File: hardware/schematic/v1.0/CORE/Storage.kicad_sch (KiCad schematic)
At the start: 43 parts, among them J12 USB_C_Receptacle_USB2.0_16P, U1 TXS02612RTWR, U12 FT2232HL, U3 SD_Card, U6 93LC56BT-I_OT, X1 X322512MSB4SI

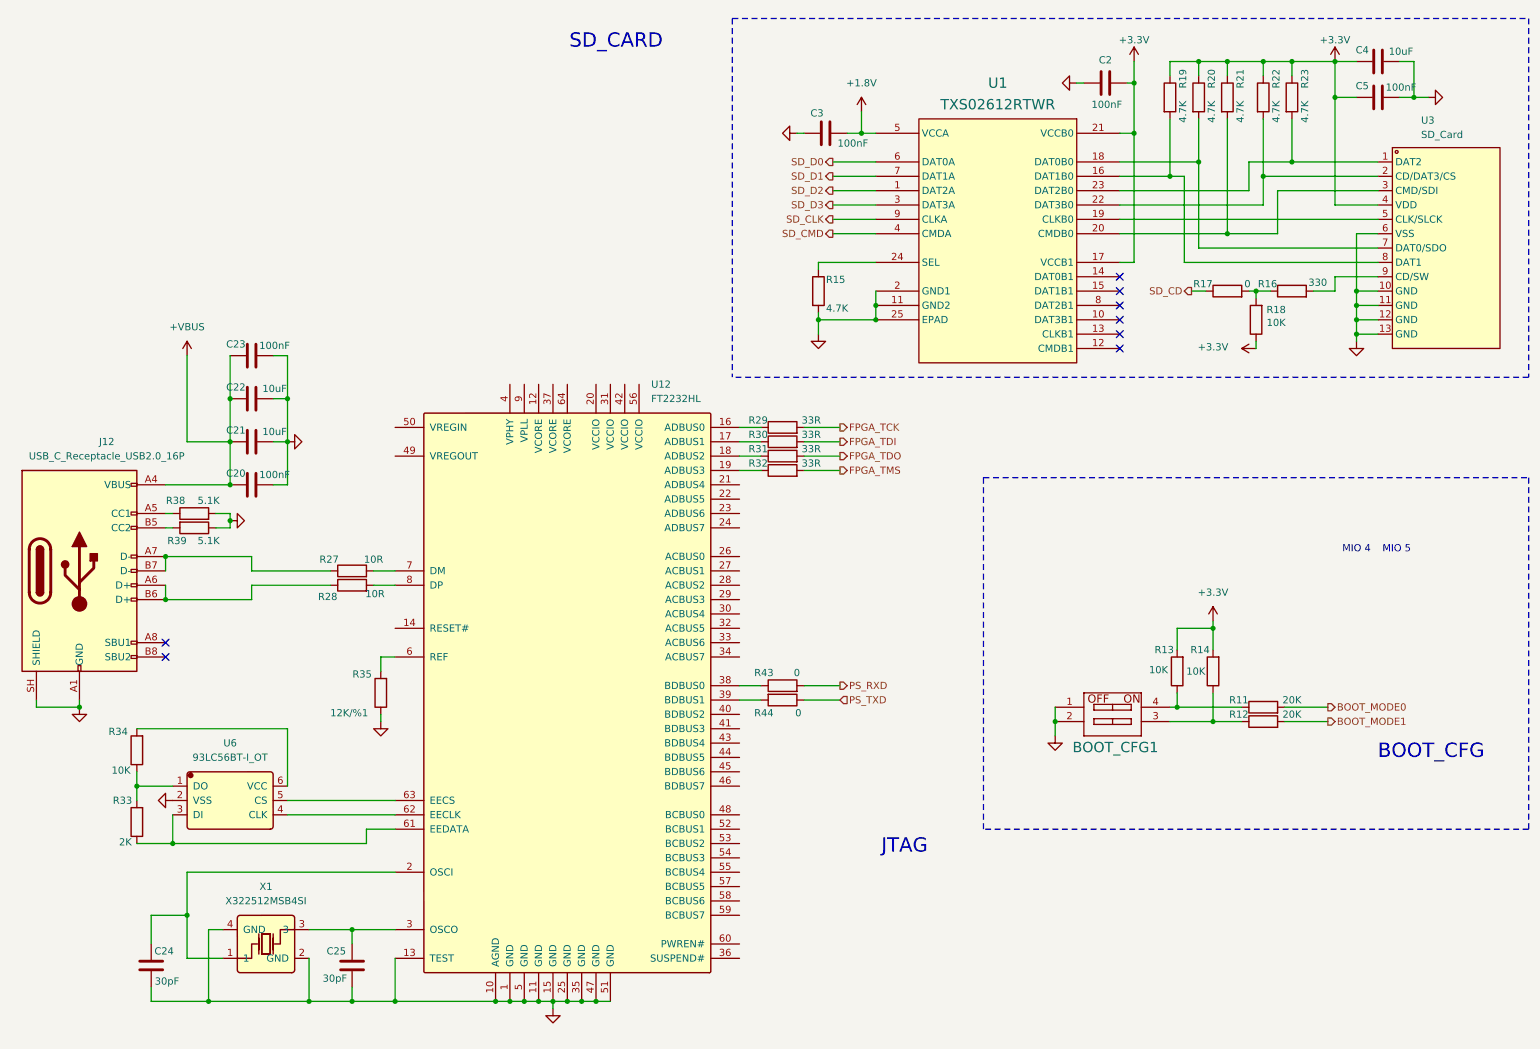
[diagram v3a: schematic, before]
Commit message: sch update
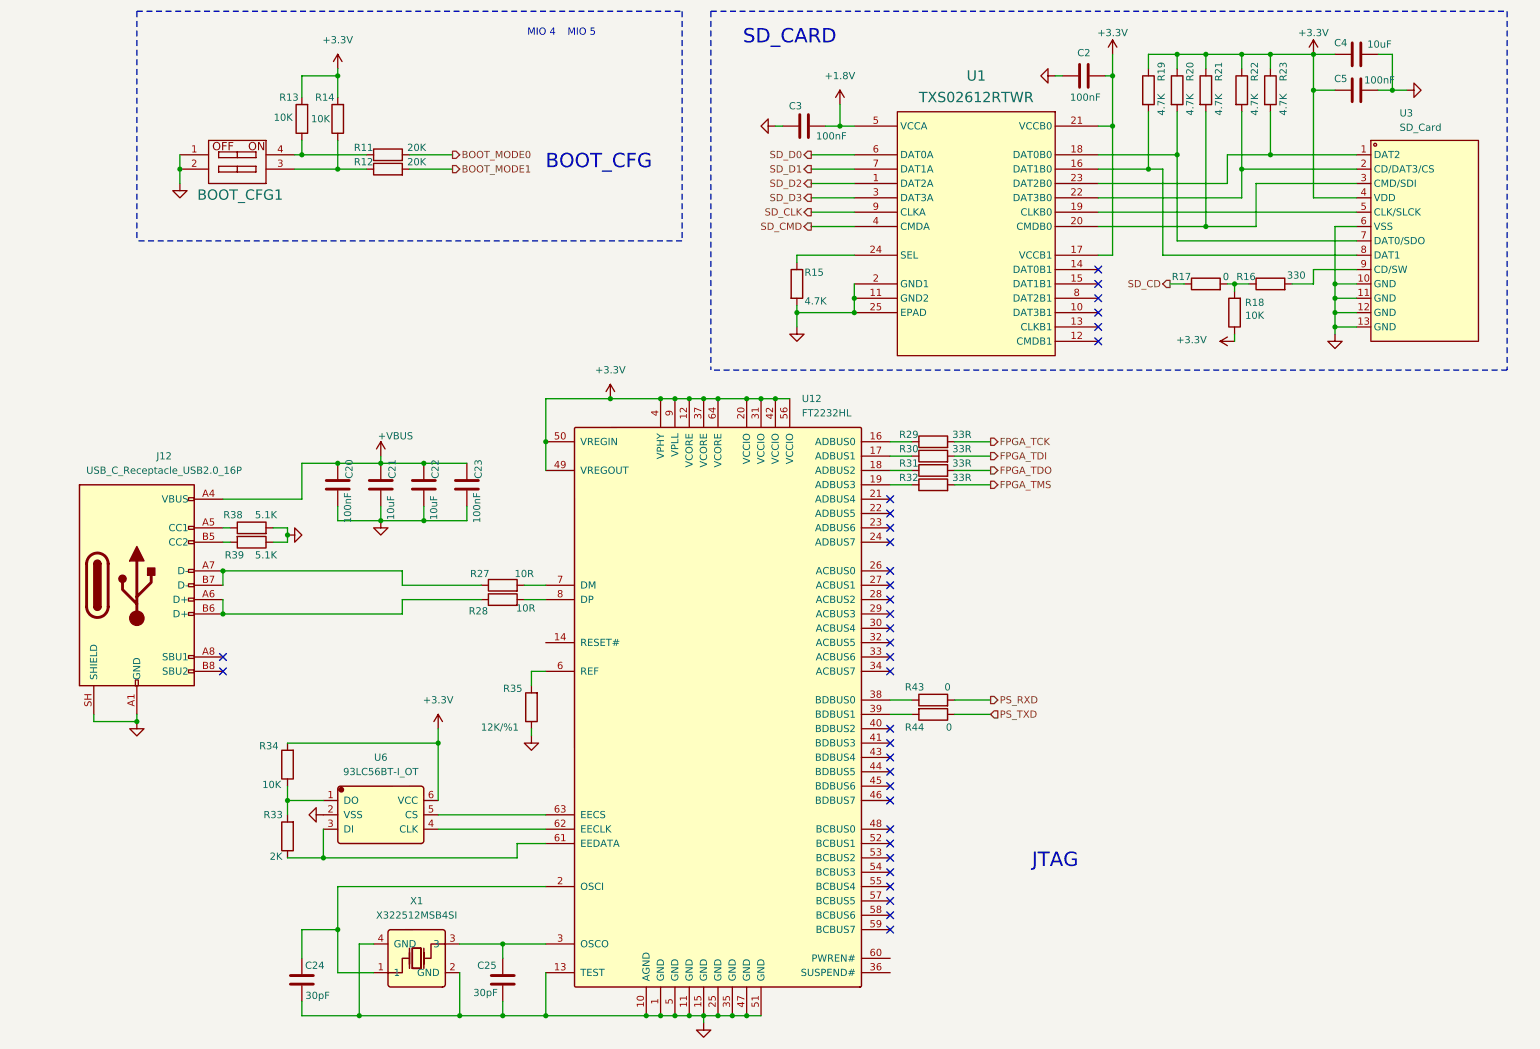
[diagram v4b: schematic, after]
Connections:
- net +3.3V: now also R34.2, U12.12 (VCORE), U12.20 (VCCIO), U12.31 (VCCIO), U12.37 (VCORE), U12.4 (VPHY), U12.42 (VCCIO), U12.49 (VREGOUT), U12.50 (VREGIN), U12.56 (VCCIO), U12.64 (VCORE), U12.9 (VPLL), U6.6 (VCC)
- no-connect marks 8 -> 34
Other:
- moved on the sheet: BOOT_CFG1, C2, C20, C21, C22, C23, C24, C25, C3, C4, C5, J12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
